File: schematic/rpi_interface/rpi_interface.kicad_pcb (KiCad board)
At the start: 2 copper layers, 30 parts, among them P1 CONN_01X04, P2 CONN_01X06, P3 CONN_01X03, U1 MCT6, U2 MCT6, U3 MCT6, U4 MCT6, U5 ULN2003, U6 Raspberry_Pi_2_3

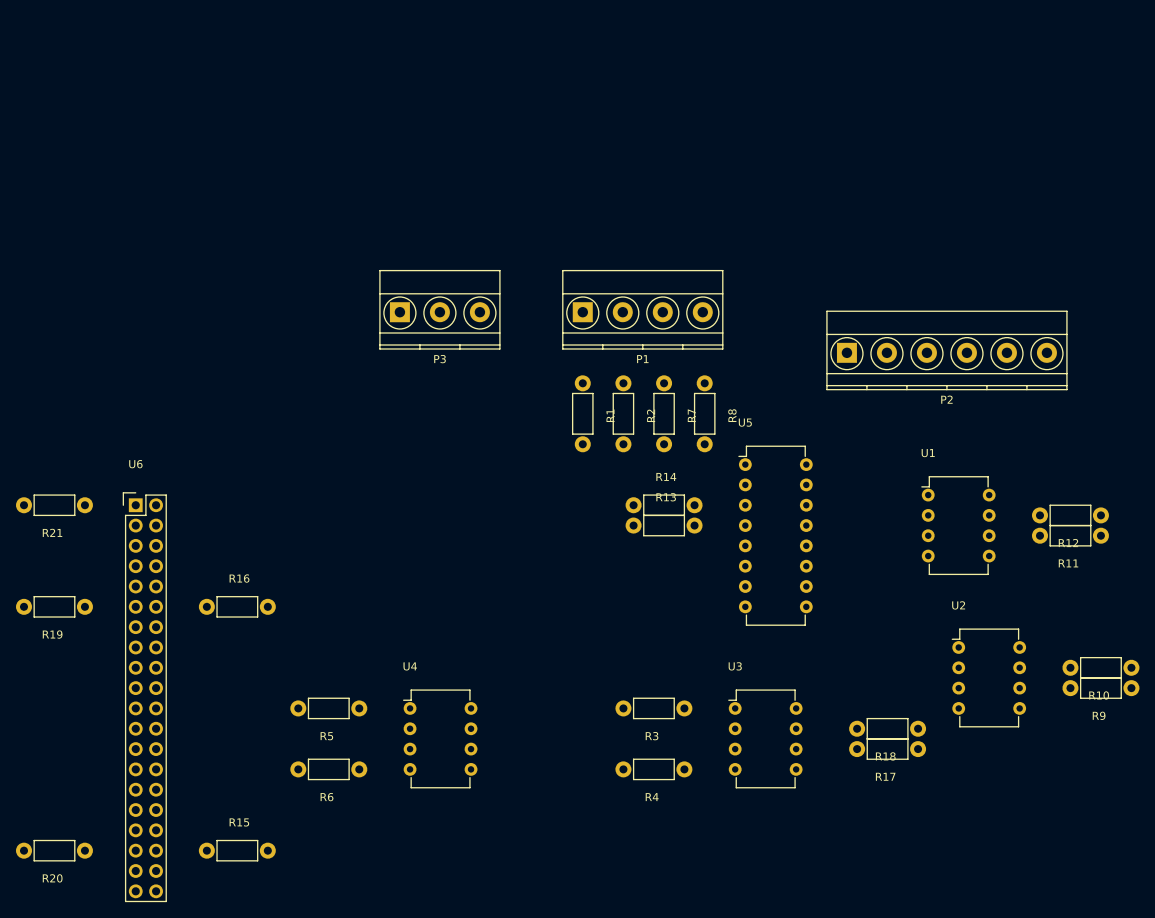
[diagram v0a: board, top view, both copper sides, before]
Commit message: Worked out how to iterate wvalue array
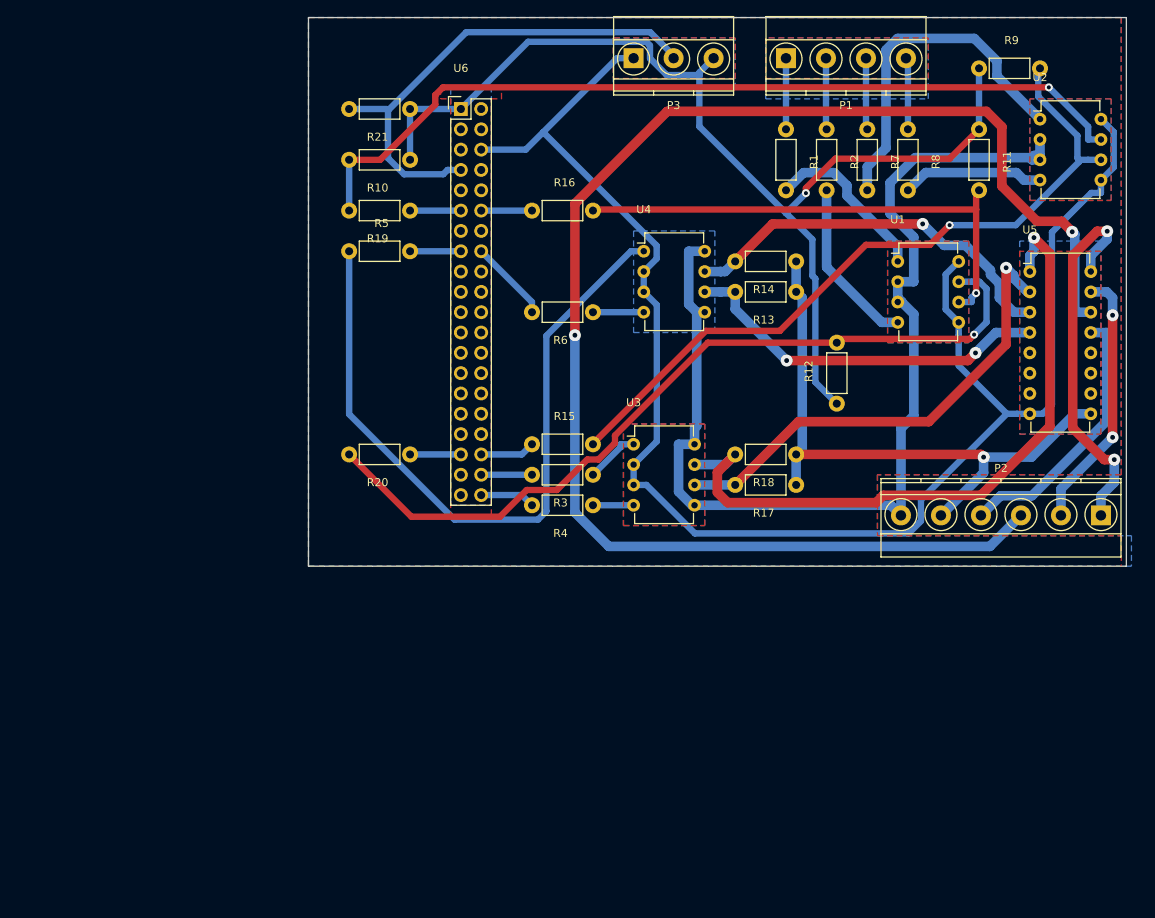
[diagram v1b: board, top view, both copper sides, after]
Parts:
- moved R10 110.3 mm to (130.8, 67.3)
- moved R9 79.8 mm to (201.9, 55.9), turned to 0 degrees
- moved U2 66.8 mm to (209.6, 62.2)
- moved R15 65.1 mm to (146.1, 102.9)
- moved U4 64.2 mm to (160.0, 78.7)
- moved R6 64.2 mm to (153.7, 86.4)
- moved R16 64.1 mm to (146.1, 73.7)
- moved R19 64.1 mm to (130.8, 73.7)
- moved R20 64.1 mm to (130.8, 104.1)
- moved R21 64.1 mm to (130.8, 61.0)
- moved U6 64.1 mm to (137.2, 61.0)
- moved R5 57.2 mm to (123.2, 78.7), turned to 0 degrees
- moved R11 53.0 mm to (201.9, 63.5), turned to 270 degrees
- moved P3 43.1 mm to (158.8, 54.6)
- moved U5 43.0 mm to (208.3, 81.3)
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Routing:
- net GND: track 0.00 -> 202.5 mm
- net Net-(P2-Pad3): track 0.00 -> 187.4 mm, vias 0 -> 2
- net +3V3: track 0.00 -> 136.1 mm, vias 0 -> 1
- net GNDA: track 0.00 -> 134.8 mm
- net Net-(R10-Pad2): track 0.00 -> 108.4 mm, vias 0 -> 1
- net Net-(R12-Pad2): track 0.00 -> 101.5 mm, vias 0 -> 1
- net Net-(R15-Pad2): track 0.00 -> 92.1 mm, vias 0 -> 1
- net Net-(R5-Pad1): track 0.00 -> 89.4 mm
- net Net-(R18-Pad2): track 0.00 -> 86.2 mm, vias 0 -> 1
- net +24V: track 0.00 -> 77.3 mm, vias 0 -> 1
- net Net-(R11-Pad2): track 0.00 -> 63.9 mm, vias 0 -> 1
- net Net-(P3-Pad2): track 0.00 -> 62.4 mm
- net Net-(R17-Pad2): track 0.00 -> 60.2 mm, vias 0 -> 1
- net Net-(R14-Pad2): track 0.00 -> 49.0 mm, vias 0 -> 1
- net Net-(P2-Pad1): track 0.00 -> 47.5 mm, vias 0 -> 2
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- added copper zone on B.Cu, net (none)
- added copper zone on F.Cu, net (none)
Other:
- board outline added: 102.2 x 68.6 mm
- net class 24v added: clearance 0.6, trace_width 1.2, via_dia 1.5, via_drill 0.6
- net class Default: clearance 0.2 -> 0.4; trace_width 0.25 -> 0.8; via_dia 0.6 -> 1; via_drill 0.4 -> 0.6
- rule trace_clearance: 0.2 -> 0.4
